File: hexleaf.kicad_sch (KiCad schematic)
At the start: 53 parts, among them IC1 ESP32-C3-FH4, IC2 MAX14781EESA+, J1 009155005201006, J2 Conn_01x04, J3 009155005201006, J5 Conn_01x08, J6 Conn_01x04, J7 Conn_01x08, SW1 SW_SPST, SW2 SW_SPST, Y1 ECS-400-10-37B2-CKM-TR

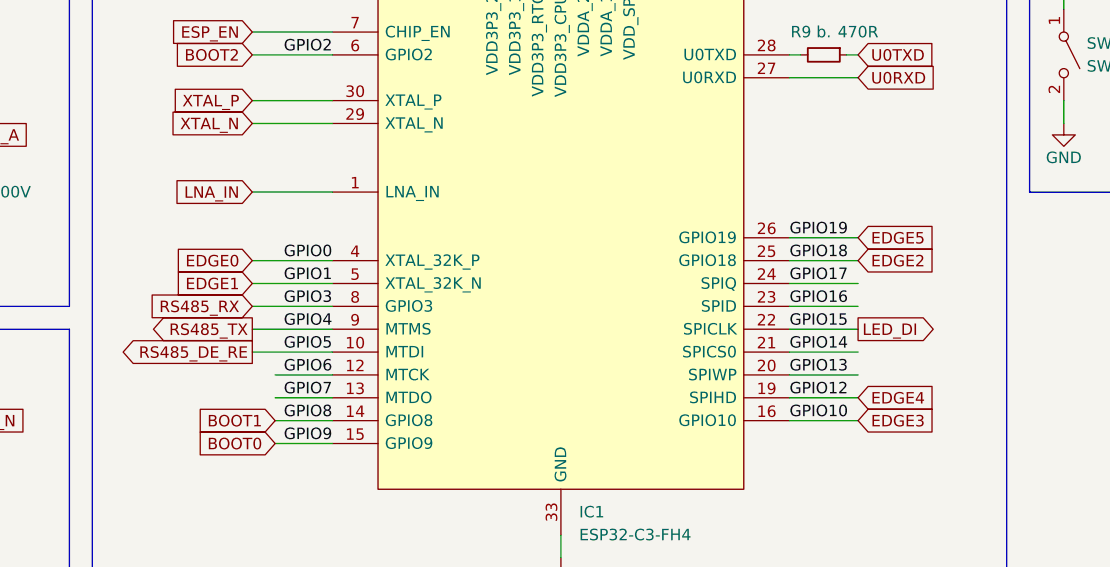
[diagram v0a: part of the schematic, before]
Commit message: started layout
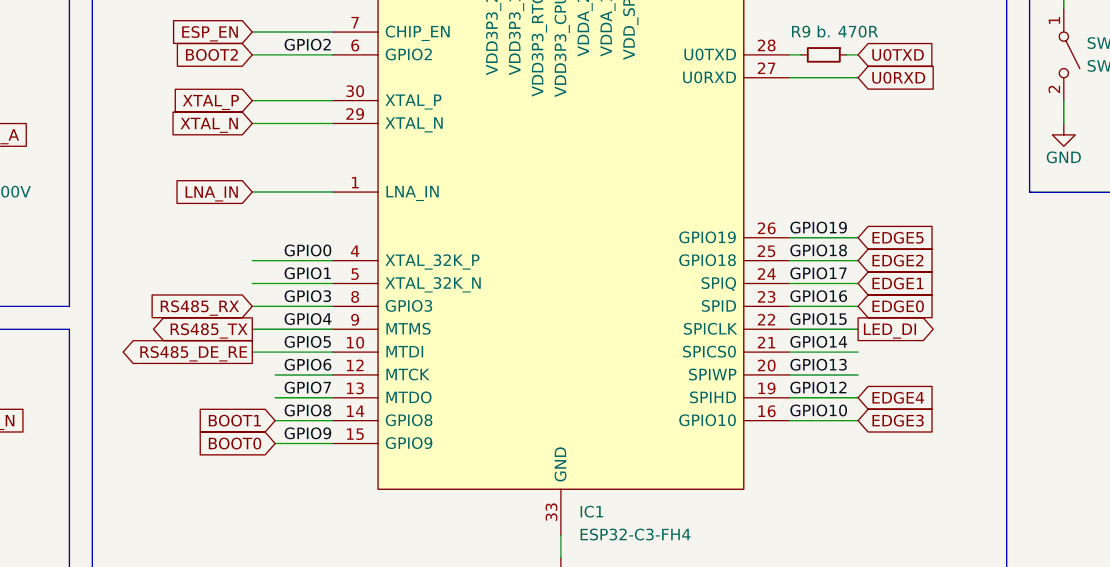
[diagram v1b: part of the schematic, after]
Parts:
- J6: footprint (none) -> hexleaf:WS2815_Strip_4P_Full
- R12, R13: footprint Resistor_SMD:R_0805_2012Metric -> Resistor_SMD:R_0402_1005Metric
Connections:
- net GPIO16 is gone; now on net EDGE0: IC1.23 (SPID)
- net GPIO17 is gone; now on net EDGE1: IC1.24 (SPIQ)
- net EDGE0: no longer IC1.4 (XTAL_32K_P)
- net EDGE1: no longer IC1.5 (XTAL_32K_N)
- new net GPIO0: IC1.4 (XTAL_32K_P)
- new net GPIO1: IC1.5 (XTAL_32K_N)
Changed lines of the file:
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@@
     )
   )
-  (global_label "EDGE1" (shape input) (at 259.08 86.36 180) (fields_autoplaced)
-    (effects (font (size 1.27 1.27)) (justify right))
-    (property "Intersheet References" "${INTERSHEET_REFS}" (id 0) (at 250.7082 86.2806 0)
-      (effects (font (size 1.27 1.27)) (justify right) hide)
+  (global_label "EDGE1" (shape input) (at 326.39 86.36 0) (fields_autoplaced)
+    (effects (font (size 1.27 1.27)) (justify left))
+    (property "Intersheet References" "${INTERSHEET_REFS}" (id 0) (at 334.7618 86.4394 0)
+      (effects (font (size 1.27 1.27)) (justify left) hide)
     )
   )
@@
     )
   )
-  (global_label "EDGE0" (shape input) (at 259.08 83.82 180) (fields_autoplaced)
-    (effects (font (size 1.27 1.27)) (justify right))
-    (property "Intersheet References" "${INTERSHEET_REFS}" (id 0) (at 250.7082 83.7406 0)
-      (effects (font (size 1.27 1.27)) (justify right) hide)
+  (global_label "EDGE0" (shape input) (at 326.39 88.9 0) (fields_autoplaced)
+    (effects (font (size 1.27 1.27)) (justify left))
+    (property "Intersheet References" "${INTERSHEET_REFS}" (id 0) (at 334.7618 88.9794 0)
+      (effects (font (size 1.27 1.27)) (justify left) hide)
     )
   )
@@
     (property "Reference" "R13" (id 0) (at 382.27 59.69 0))
     (property "Value" "10k" (id 1) (at 382.27 62.23 0))
-    (property "Footprint" "Resistor_SMD:R_0805_2012Metric" (id 2) (at 378.46 60.96 0)
+    (property "Footprint" "Resistor_SMD:R_0402_1005Metric" (id 2) (at 378.46 60.96 0)
       (effects (font (size 1.27 1.27)) hide)
     )
@@
       (effects (font (size 1.27 1.27)) (justify left))
     )
-    (property "Footprint" "" (id 2) (at 106.68 149.86 0)
+    (property "Footprint" "hexleaf:WS2815_Strip_4P_Full" (id 2) (at 106.68 149.86 0)
       (effects (font (size 1.27 1.27)) hide)
     )
@@
     (property "Datasheet" "~" (id 3) (at 284.48 157.48 0)
       (effects (font (size 1.27 1.27)) hide)
+    )
+    (pin "1")
+    (pin "2")
+  )
+  (symbol (lib_id "Device:R_Small") (at 378.46 40.64 180) (unit 1)
+    (in_bom yes) (on_board yes)
+    (property "Reference" "R12" (id 0) (at 382.27 39.37 0))
+    (property "Value" "10k" (id 1) (at 382.27 41.91 0))
+    (property "Footprint" "Resistor_SMD:R_0402_1005Metric" (id 2) (at 378.46 40.64 0)
+      (effects (font (size 1.27 1.27)) hide)
+    )
+    (property "Datasheet" "https://www.mouser.de/datasheet/2/447/PYu_RC_Group_51_RoHS_L_10-1664068.pdf" (id 3) (at 378.46 40.64 0)
+      (effects (font (size 1.27 1.27)) hide)
+    )
+    (property "MFN" " 603-RC0402FR-0710KL " (id 4) (at 378.46 40.64 0)
+      (effects (font (size 1.27 1.27)) hide)
+    )
+    (property "in stock" "b." (id 5) (at 377.19 40.64 0)
+      (effects (font (size 1.27 1.27)) (justify left))
     )
     (pin "1")
@@
     (pin "2")
   )
-  (symbol (lib_id "Device:R_Small") (at 378.46 40.64 180) (unit 1)
-    (in_bom yes) (on_board yes)
-    (property "Reference" "R12" (id 0) (at 382.27 39.37 0))
-    (property "Value" "10k" (id 1) (at 382.27 41.91 0))
-    (property "Footprint" "Resistor_SMD:R_0805_2012Metric" (id 2) (at 378.46 40.64 0)
-      (effects (font (size 1.27 1.27)) hide)
-    )
-    (property "Datasheet" "https://www.mouser.de/datasheet/2/447/PYu_RC_Group_51_RoHS_L_10-1664068.pdf" (id 3) (at 378.46 40.64 0)
-      (effects (font (size 1.27 1.27)) hide)
-    )
-    (property "MFN" " 603-RC0402FR-0710KL " (id 4) (at 378.46 40.64 0)
-      (effects (font (size 1.27 1.27)) hide)
-    )
-    (property "in stock" "b." (id 5) (at 377.19 40.64 0)
-      (effects (font (size 1.27 1.27)) (justify left))
-    )
-    (pin "1")
-    (pin "2")
-  )
   (symbol (lib_id "Jumper:SolderJumper_2_Open") (at 57.15 152.4 90) (unit 1)
     (in_bom yes) (on_board yes)
@@
     )
     (path "/16e7f86d-2283-4e9b-86c9-30f5f38f682b"
-      (reference "J6") (unit 1) (value "Conn_01x04") (footprint "")
+      (reference "J6") (unit 1) (value "Conn_01x04") (footprint "hexleaf:WS2815_Strip_4P_Full")
     )
     (path "/28d5f755-ae65-42a6-882e-df3c414cf483"
@@
       (reference "R11") (unit 1) (value "470R") (footprint "Resistor_SMD:R_0402_1005Metric")
     )
-    (path "/eb0bb8bc-b294-4a58-a337-95a413bdd34a"
-      (reference "R12") (unit 1) (value "10k") (footprint "Resistor_SMD:R_0805_2012Metric")
+    (path "/8208a877-1896-47c5-b498-a9a96b7a0534"
+      (reference "R12") (unit 1) (value "10k") (footprint "Resistor_SMD:R_0402_1005Metric")
     )
     (path "/0a517b9a-a9fc-44f0-b6e1-5b5bad5d4c74"
-      (reference "R13") (unit 1) (value "10k") (footprint "Resistor_SMD:R_0805_2012Metric")
+      (reference "R13") (unit 1) (value "10k") (footprint "Resistor_SMD:R_0402_1005Metric")
     )
     (path "/508cc352-4d19-4358-95ba-715645cd1a5a"
